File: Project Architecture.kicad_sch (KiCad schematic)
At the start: 0 parts

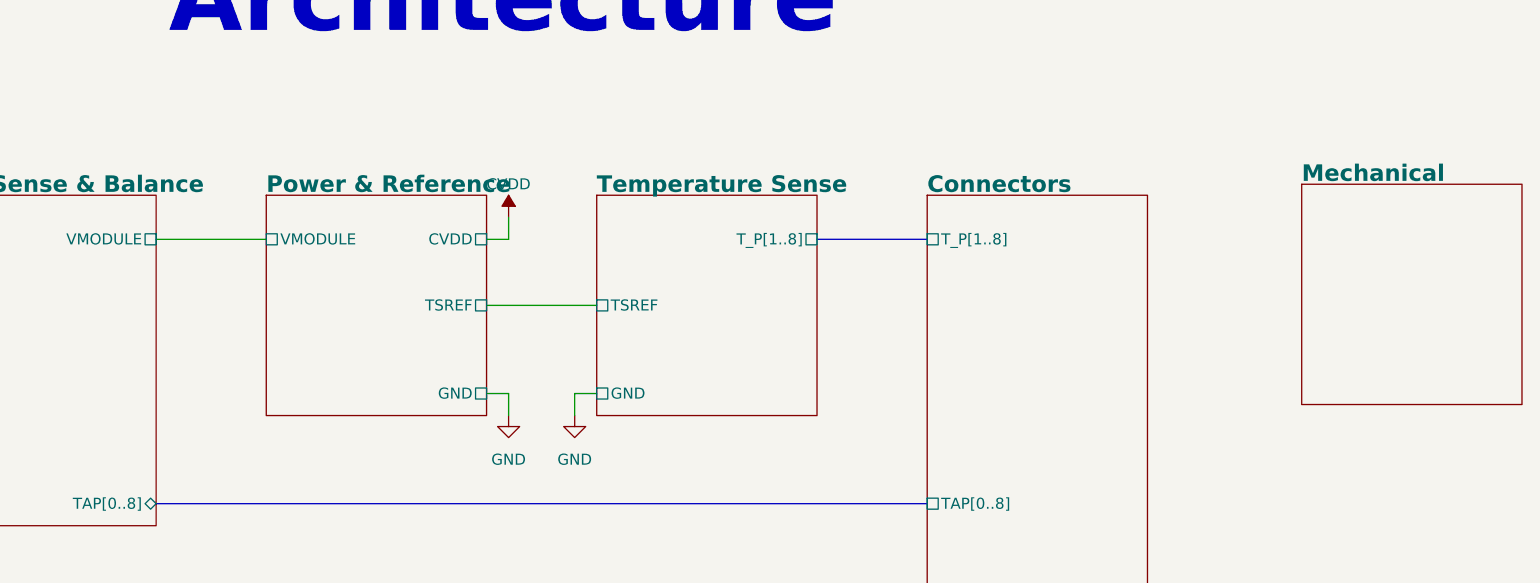
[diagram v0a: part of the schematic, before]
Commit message: SCH[Cleaning]:Updated Connectors not sure still, added sprate bat and ground connections, updated commincation conncetors. PCB[Layout]:Inital layout of compents need to fit on board size once tap connecton method is decided.
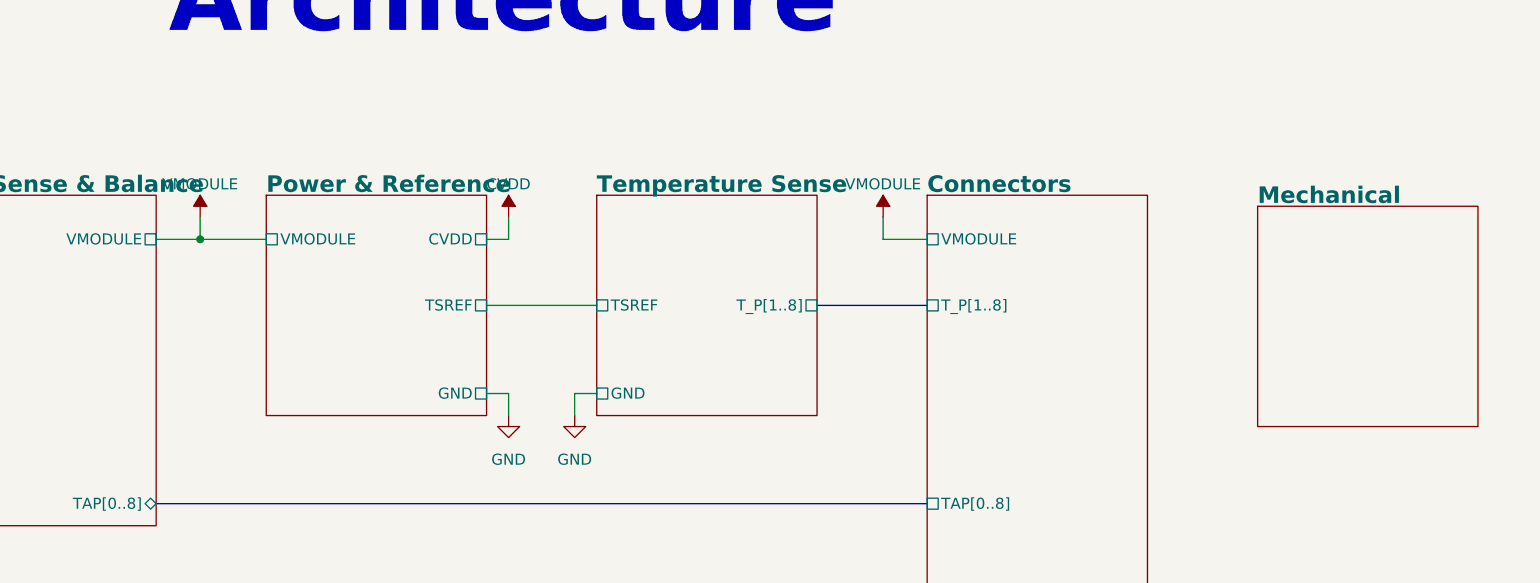
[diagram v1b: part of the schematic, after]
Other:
- sheet Connectors ports: added VMODULE; removed none
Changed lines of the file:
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@@
 	(title_block
 		(title "Project Architecture")
-		(date "2025-01-12")
 		(rev "${REVISION}")
 		(company "${COMPANY}")
@@
 		)
 	)
+	(junction
+		(at 106.68 60.96)
+		(diameter 0)
+		(color 0 0 0 0)
+	)
 	(wire
 		(pts
@@
 		)
 	)
+	(wire
+		(pts
+			(xy 185.42 58.42) (xy 185.42 60.96)
+		)
+		(stroke
+			(width 0)
+			(type default)
+		)
+	)
 	(bus
 		(pts
@@
 	(wire
 		(pts
+			(xy 185.42 60.96) (xy 190.5 60.96)
+		)
+		(stroke
+			(width 0)
+			(type default)
+		)
+	)
+	(wire
+		(pts
 			(xy 190.5 129.54) (xy 187.96 129.54)
 		)
@@
 	(wire
 		(pts
+			(xy 106.68 60.96) (xy 114.3 60.96)
+		)
+		(stroke
+			(width 0)
+			(type default)
+		)
+	)
+	(wire
+		(pts
 			(xy 187.96 129.54) (xy 187.96 132.08)
 		)
@@
 	(bus
 		(pts
-			(xy 177.8 60.96) (xy 190.5 60.96)
+			(xy 177.8 68.58) (xy 190.5 68.58)
 		)
 		(stroke
@@
 	(wire
 		(pts
-			(xy 101.6 60.96) (xy 114.3 60.96)
+			(xy 101.6 60.96) (xy 106.68 60.96)
 		)
 		(stroke
@@
 		(pts
 			(xy 152.4 78.74) (xy 149.86 78.74)
+		)
+		(stroke
+			(width 0)
+			(type default)
+		)
+	)
+	(wire
+		(pts
+			(xy 106.68 58.42) (xy 106.68 60.96)
 		)
 		(stroke
@@
 	)
 	(symbol
+		(lib_id "power:VSSA")
+		(at 106.68 58.42 0)
+		(unit 1)
+		(body_style 1)
+		(exclude_from_sim no)
+		(in_bom yes)
+		(on_board yes)
+		(in_pos_files yes)
+		(dnp no)
+		(property "Reference" "#PWR054"
+			(at 106.68 62.23 0)
+			(hide yes)
+			(show_name no)
+			(do_not_autoplace no)
+			(effects
+				(font
+					(size 1.27 1.27)
+				)
+			)
+		)
+		(property "Value" "VMODULE"
+			(at 106.68 54.61 0)
+			(show_name no)
+			(do_not_autoplace no)
+			(effects
+				(font
+					(size 1.27 1.27)
+				)
+			)
+		)
+		(property "Footprint" ""
+			(at 106.68 58.42 0)
+			(hide yes)
+			(show_name no)
+			(do_not_autoplace no)
+			(effects
+				(font
+					(size 1.27 1.27)
+				)
+			)
+		)
+		(property "Datasheet" ""
+			(at 106.68 58.42 0)
+			(hide yes)
+			(show_name no)
+			(do_not_autoplace no)
+			(effects
+				(font
+					(size 1.27 1.27)
+				)
+			)
+		)
+		(property "Description" "Power symbol creates a local label with name \"VSSA\""
+			(at 106.68 58.42 0)
+			(hide yes)
+			(show_name no)
+			(do_not_autoplace no)
+			(effects
+				(font
+					(size 1.27 1.27)
+				)
+			)
+		)
+		(pin "1"
+		)
+		(instances
+			(project "bms_slave"
+				(path "/f9e05184-c88b-4a88-ae9c-ab2bdb32be7c/c5103ceb-5325-4a84-a025-9638a412984e"
+					(reference "#PWR054")
+					(unit 1)
+				)
+			)
+		)
+	)
+	(symbol
 		(lib_id "power:GND")
 		(at 149.86 81.28 0)
@@
 		)
 	)
+	(symbol
+		(lib_id "power:VSSA")
+		(at 185.42 58.42 0)
+		(unit 1)
+		(body_style 1)
+		(exclude_from_sim no)
+		(in_bom yes)
+		(on_board yes)
+		(in_pos_files yes)
+		(dnp no)
+		(property "Reference" "#PWR055"
+			(at 185.42 62.23 0)
+			(hide yes)
+			(show_name no)
+			(do_not_autoplace no)
+			(effects
+				(font
+					(size 1.27 1.27)
+				)
+			)
+		)
+		(property "Value" "VMODULE"
+			(at 185.42 54.61 0)
+			(show_name no)
+			(do_not_autoplace no)
+			(effects
+				(font
+					(size 1.27 1.27)
+				)
+			)
+		)
+		(property "Footprint" ""
+			(at 185.42 58.42 0)
+			(hide yes)
+			(show_name no)
+			(do_not_autoplace no)
+			(effects
+				(font
+					(size 1.27 1.27)
+				)
+			)
+		)
+		(property "Datasheet" ""
+			(at 185.42 58.42 0)
+			(hide yes)
+			(show_name no)
+			(do_not_autoplace no)
+			(effects
+				(font
+					(size 1.27 1.27)
+				)
+			)
+		)
+		(property "Description" "Power symbol creates a local label with name \"VSSA\""
+			(at 185.42 58.42 0)
+			(hide yes)
+			(show_name no)
+			(do_not_autoplace no)
+			(effects
+				(font
+					(size 1.27 1.27)
+				)
+			)
+		)
+		(pin "1"
+		)
+		(instances
+			(project "bms_slave"
+				(path "/f9e05184-c88b-4a88-ae9c-ab2bdb32be7c/c5103ceb-5325-4a84-a025-9638a412984e"
+					(reference "#PWR055")
+					(unit 1)
+				)
+			)
+		)
+	)
 	(sheet
 		(at 152.4 55.88)
@@
 		)
 		(pin "T_P[1..8]" passive
-			(at 177.8 60.96 0)
+			(at 177.8 68.58 0)
 			(effects
 				(font
@@
 		)
 		(pin "T_P[1..8]" passive
-			(at 190.5 60.96 180)
+			(at 190.5 68.58 180)
 			(effects
 				(font
@@
 					(size 1.27 1.27)
 					(color 0 0 0 1)
+				)
+				(justify left)
+			)
+		)
+		(pin "VMODULE" passive
+			(at 190.5 60.96 180)
+			(effects
+				(font
+					(size 1.27 1.27)
 				)
 				(justify left)
@@
 	)
 	(sheet
-		(at 233.68 54.61)
+		(at 228.6 57.15)
 		(size 25.4 25.4)
 		(exclude_from_sim no)
@@
 		)
 		(fill
-			(color 0 0 0 0)
+			(color 255 255 194 1)
 		)
 		(property "Sheetname" "Mechanical"
-			(at 233.68 53.34 0)
+			(at 228.6 55.88 0)
 			(show_name no)
 			(do_not_autoplace no)
@@
 		)
 		(property "Sheetfile" "mechanical.kicad_sch"
-			(at 233.68 80.5946 0)
-			(hide yes)
-			(show_name no)
+			(at 228.6 83.1346 0)
+			(hide yes)
+			(show_name no)
